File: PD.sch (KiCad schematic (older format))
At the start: 0 parts

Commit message: powersupply
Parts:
- added C? (x3): 0.1uF, Capacitor_SMD:C_0603_1608Metric, symbol Device:C_Small
- added C?: 1.0uF, Capacitor_SMD:C_0603_1608Metric, symbol Device:C_Small
- added R?: 16.9Ohm, Resistor_SMD:R_0603_1608Metric, symbol Device:R_Small
- added R? (x3): 0Ohm, Resistor_SMD:R_0603_1608Metric, symbol Device:R_Small
- added R?: 20Ohm, Resistor_SMD:R_0603_1608Metric, symbol Device:R_Small
- added R?: 37.4KOhm, Resistor_SMD:R_0603_1608Metric, symbol Device:R_Small
- added R?: 12.1KOhm, Resistor_SMD:R_0603_1608Metric, symbol Device:R_Small
- added R? (x2): 1.91KOhm, Resistor_SMD:R_0603_1608Metric, symbol Device:R_Small
- added R? (x3): 69.8Ohm, Resistor_SMD:R_0603_1608Metric, symbol Device:R_Small
- added U?: ISL95837HRZ-T, Package_DFN_QFN:QFN-40-1EP_6x6mm_P0.5mm_EP4.6x4.6mm, symbol ISL95837:ISL95837HRZ-T
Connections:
- new net: R?.1, U?.2 (PGOODG)
- new net: R?.1, U?.3 (SDA)
- new net: R?.1, U?.4 (ALERT#)
- new net: R?.1, U?.5 (SCLK)
- new net: C?.1, R?.1, R?.2, U?.6 (VR_ON)
- new net: R?.1, U?.7 (PGOOD)
- new net +1V0: C?.1, R?.1, R?.1, R?.1
- new net +3V3: R?.2, R?.2
- new net GFX_PG: C?.1, R?.1, R?.2
- new net GND: C?.2, C?.2, C?.2, C?.2, R?.2
- new net SVID_ALERT-R: R?.2, R?.2
- new net SVID_CLK-R: R?.2, R?.2
- new net SVID_DATA-R: R?.2, R?.2
- new net VCC: R?.1
- new net VCORE_PG: C?.1, R?.1, R?.2
- new net VR_HOT_L: U?.8 (VR_HOT#)

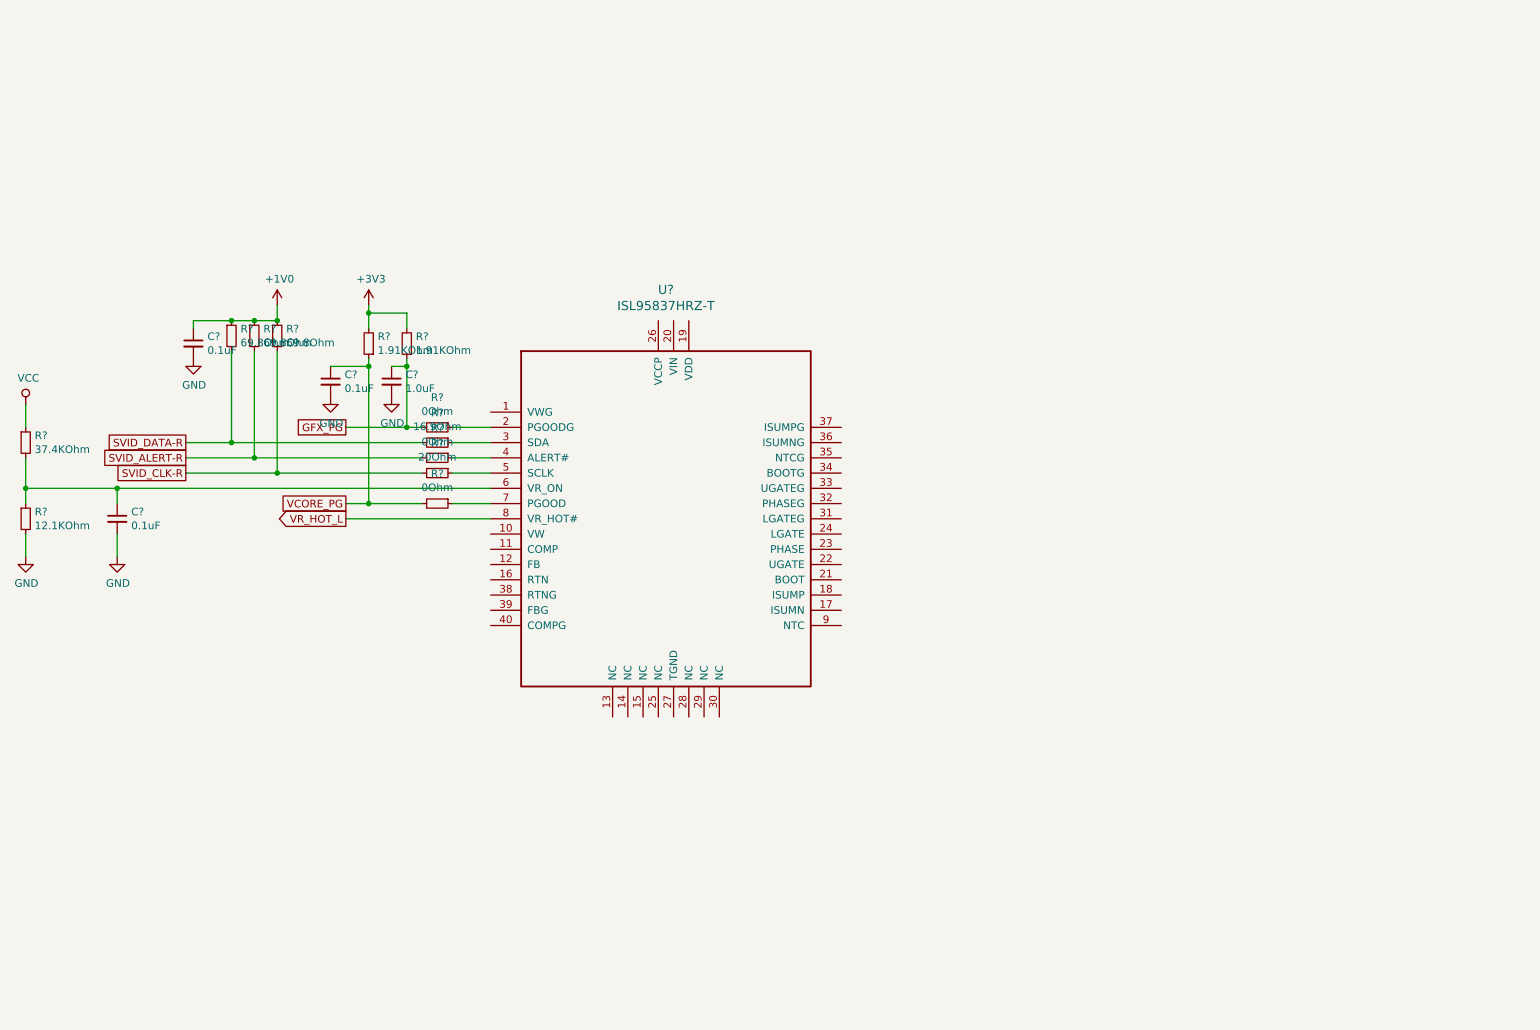
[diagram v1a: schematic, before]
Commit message: rest of power controller
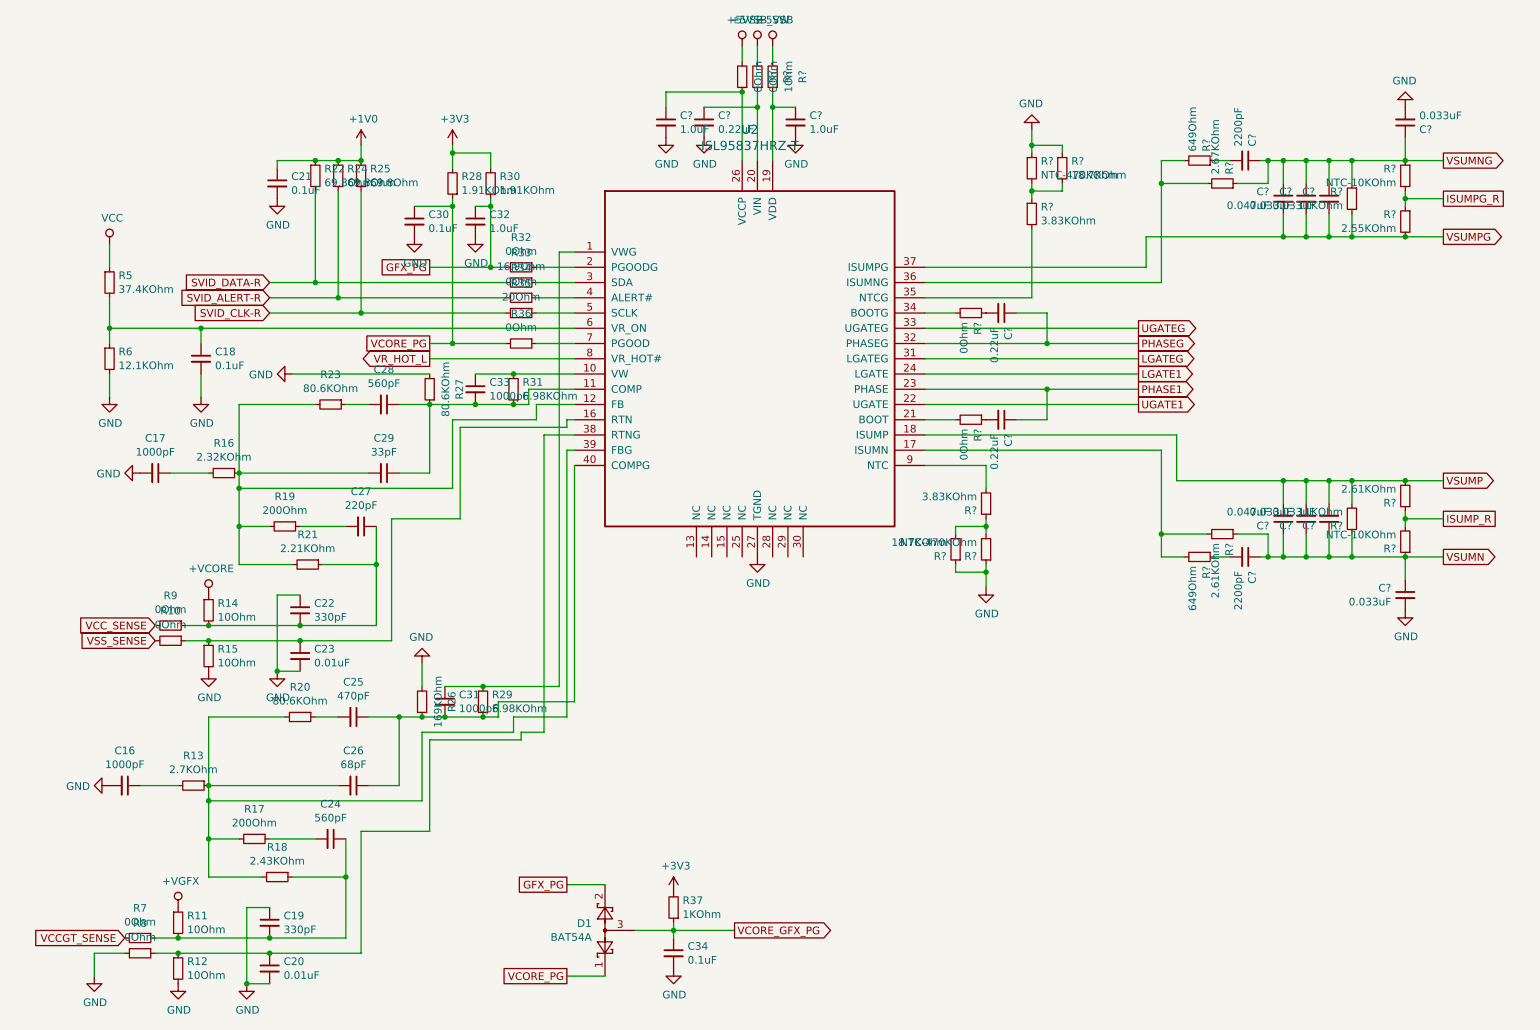
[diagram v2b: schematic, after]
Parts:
- added C16, C17, C31, C33: 1000pF, Capacitor_SMD:C_0603_1608Metric, symbol Device:C_Small
- added C19, C22: 330pF, Capacitor_SMD:C_0603_1608Metric, symbol Device:C_Small
- added C20, C23: 0.01uF, Capacitor_SMD:C_0603_1608Metric, symbol Device:C_Small
- added C24, C28: 560pF, Capacitor_SMD:C_0603_1608Metric, symbol Device:C_Small
- added C25: 470pF, Capacitor_SMD:C_0603_1608Metric, symbol Device:C_Small
- added C26: 68pF, Capacitor_SMD:C_0603_1608Metric, symbol Device:C_Small
- added C27: 220pF, Capacitor_SMD:C_0603_1608Metric, symbol Device:C_Small
- added C29: 33pF, Capacitor_SMD:C_0603_1608Metric, symbol Device:C_Small
- added C34: 0.1uF, Capacitor_SMD:C_0603_1608Metric, symbol Device:C_Small
- added C? (x3): 0.22uF, Capacitor_SMD:C_0603_1608Metric, symbol Device:C_Small
- added C? (x6): 0.033uF, Capacitor_SMD:C_0603_1608Metric, symbol Device:C_Small
- added C? (x2): 0.047uF, Capacitor_SMD:C_0603_1608Metric, symbol Device:C_Small
- added C? (x2): 2200pF, Capacitor_SMD:C_0603_1608Metric, symbol Device:C_Small
- added C? (x2): 1.0uF, Capacitor_SMD:C_0603_1608Metric, symbol Device:C_Small
- added D1: BAT54A, Package_TO_SOT_SMD:SOT-23, symbol Diode:BAT54A
- added R10, R7, R8, R9, R? (x4): 0Ohm, Resistor_SMD:R_0603_1608Metric, symbol Device:R_Small
- added R11, R12, R14, R15: 10Ohm, Resistor_SMD:R_0603_1608Metric, symbol Device:R_Small
- added R13: 2.7KOhm, Resistor_SMD:R_0603_1608Metric, symbol Device:R_Small
- added R16: 2.32KOhm, Resistor_SMD:R_0603_1608Metric, symbol Device:R_Small
- added R17, R19: 200Ohm, Resistor_SMD:R_0603_1608Metric, symbol Device:R_Small
- added R18: 2.43KOhm, Resistor_SMD:R_0603_1608Metric, symbol Device:R_Small
- added R20, R23, R27: 80.6KOhm, Resistor_SMD:R_0603_1608Metric, symbol Device:R_Small
- added R21: 2.21KOhm, Resistor_SMD:R_0603_1608Metric, symbol Device:R_Small
- added R26: 169KOhm, Resistor_SMD:R_0603_1608Metric, symbol Device:R_Small
- added R29, R31: 6.98KOhm, Resistor_SMD:R_0603_1608Metric, symbol Device:R_Small
- added R37: 1KOhm, Resistor_SMD:R_0603_1608Metric, symbol Device:R_Small
- added R? (x2): 2.61KOhm, Resistor_SMD:R_0603_1608Metric, symbol Device:R_Small
- added R? (x2): NTC-10KOhm, Resistor_SMD:R_0603_1608Metric, symbol Device:R_Small
- added R? (x2): 11KOhm, Resistor_SMD:R_0603_1608Metric, symbol Device:R_Small
- added R? (x2): 649Ohm, Resistor_SMD:R_0603_1608Metric, symbol Device:R_Small
- added R?: 2.55KOhm, Resistor_SMD:R_0603_1608Metric, symbol Device:R_Small
- added R?: 2.67KOhm, Resistor_SMD:R_0603_1608Metric, symbol Device:R_Small
- added R? (x2): 3.83KOhm, Resistor_SMD:R_0603_1608Metric, symbol Device:R_Small
- added R? (x2): NTC-470KOhm, Resistor_SMD:R_0603_1608Metric, symbol Device:R_Small
- added R? (x2): 18.7KOhm, Resistor_SMD:R_0603_1608Metric, symbol Device:R_Small
- added R?: 1Ohm, Resistor_SMD:R_0603_1608Metric, symbol Device:R_Small
- gave numbers to parts that had none: 17
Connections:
- net +3V3: now also R37.2
- net GFX_PG: now also D1.2
- net GND: now also U2.27 (TGND), C16.2, C17.2, C19.1, C20.2, C22.1, C23.2, C34.2, C?.2, C?.2, C?.2, C?.2, C?.2, R12.2, R15.2, R26.2, R27.2, R8.2, R?.1, R?.1, R?.1, R?.1
- net VCORE_PG: now also D1.1
- net at U2.1 (VWG): now also C31.1, R29.2
- net at U2.10 (VW): now also C33.1, R31.2
- net at U2.11 (COMP): now also C28.1, C29.1, C33.2, R27.1, R31.1
- net at U2.12 (FB): now also C29.2, R16.1, R19.2, R21.2, R23.2
- net at U2.16 (RTN): now also C23.1, R10.1, R15.1
- net at U2.17 (ISUMN): now also R?.2, R?.2
- net VSUMP: now reaches U2.18 (ISUMP)
- net VSUMP: now also C?.2, C?.2, C?.2, R?.2, R?.2
- net at U2.19 (VDD): now also C?.1, R?.1
- net at U2.20 (VIN): now also C?.1, R?.1
- net at U2.21 (BOOT): now also R?.2
- net UGATE1: now reaches U2.22 (UGATE)
- net PHASE1: now reaches U2.23 (PHASE)
- net PHASE1: now also C?.1
- net LGATE1: now reaches U2.24 (LGATE)
- net at U2.26 (VCCP): now also C?.1, R?.1
- net LGATEG: now reaches U2.31 (LGATEG)
- net PHASEG: now reaches U2.32 (PHASEG)
- net PHASEG: now also C?.1
- net UGATEG: now reaches U2.33 (UGATEG)
- net at U2.34 (BOOTG): now also R?.2
- net at U2.35 (NTCG): now also R?.2
- net at U2.36 (ISUMNG): now also R?.2, R?.2
- net VSUMPG: now reaches U2.37 (ISUMPG)
- net VSUMPG: now also C?.2, C?.2, C?.2, R?.2, R?.2
- net at U2.38 (RTNG): now also C20.1, R12.1, R8.1
- net at U2.39 (FBG): now also C26.2, R13.1, R17.2, R18.2, R20.2
- net at U2.40 (COMPG): now also C25.1, C26.1, C31.2, R26.1, R29.1
- net at U2.9 (NTC): now also R?.2
- new net: C28.2, R23.1
- new net: C17.1, R16.2
- new net: C27.2, R19.1
- new net: C22.2, C27.1, R14.2, R21.1, R9.1
- new net: C25.2, R20.1
- new net: C16.1, R13.2
- new net: C24.2, R17.1
- new net: C19.2, C24.1, R11.2, R18.1, R7.1
- new net: C?.2, R?.1 (x4)
- new net: R?.1, R?.2, R?.2 (x2)
- new net +5VSB: R?.2, R?.2
- new net +5VSB_SW: R?.2
- new net +VCORE: R14.1
- new net +VGFX: R11.1
- new net ISUMPG_R: R?.1, R?.2
- new net ISUMP_R: R?.1, R?.2
- new net VCCGT_SENSE: R7.2
- new net VCC_SENSE: R9.2
- new net VCORE_GFX_PG: C34.1, D1.3, R37.1
- new net VSS_SENSE: R10.2
- new net VSUMN: C?.1, C?.1, C?.1, C?.1, C?.1, R?.1, R?.1, R?.1
- new net VSUMNG: C?.1, C?.1, C?.1, C?.1, C?.1, R?.1, R?.1, R?.1
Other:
- moved on the sheet: C18, C21, C30, C32, R22, R24, R25, R28, R30, R32, R33, R34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
